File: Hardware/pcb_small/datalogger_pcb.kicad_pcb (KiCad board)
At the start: 2 copper layers, 127.5 x 123.3 mm, 45 parts, among them J1 Micro_SD_Card_Det2, J2 Switch OUT, SW1 SW_Wuerth_450301014042, U1 DS3231MZ

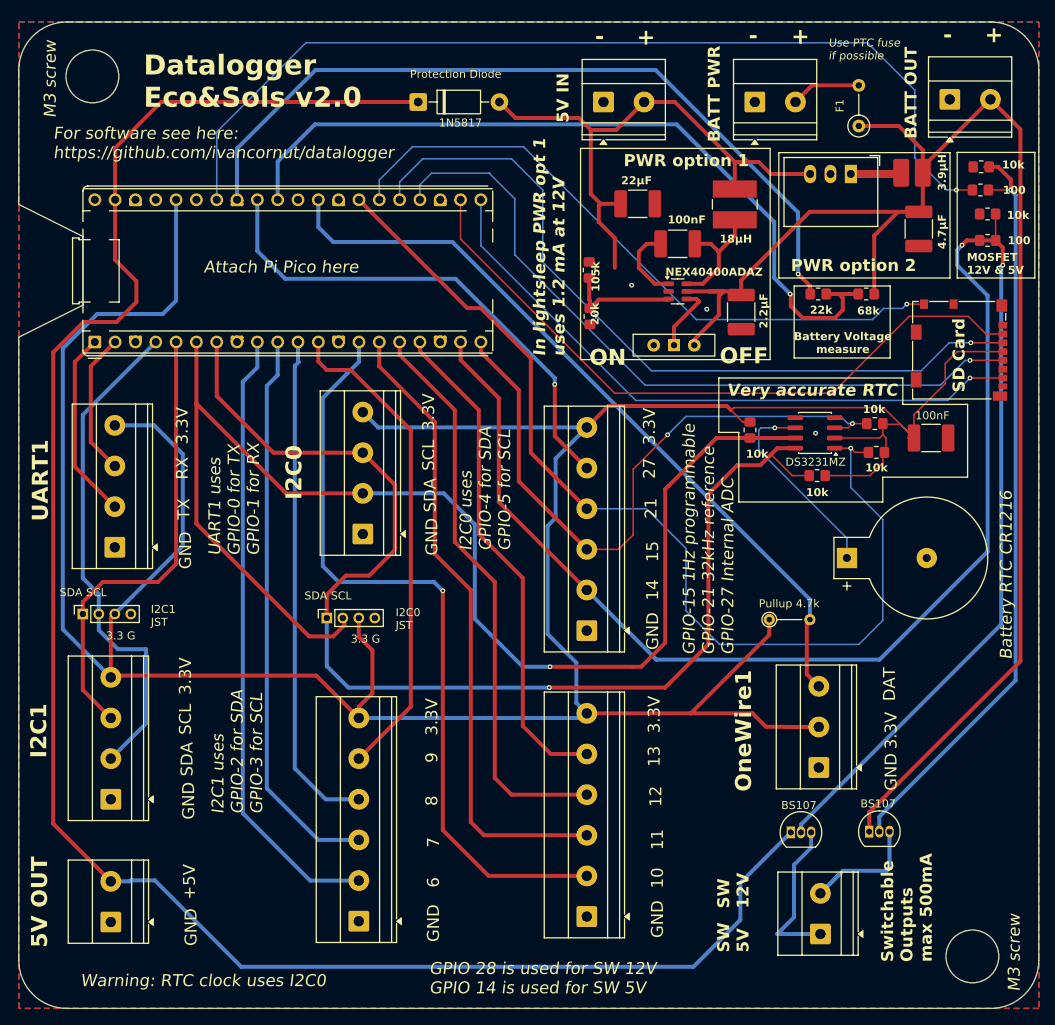
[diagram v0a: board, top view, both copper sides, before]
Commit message: Finalised design for micrologger
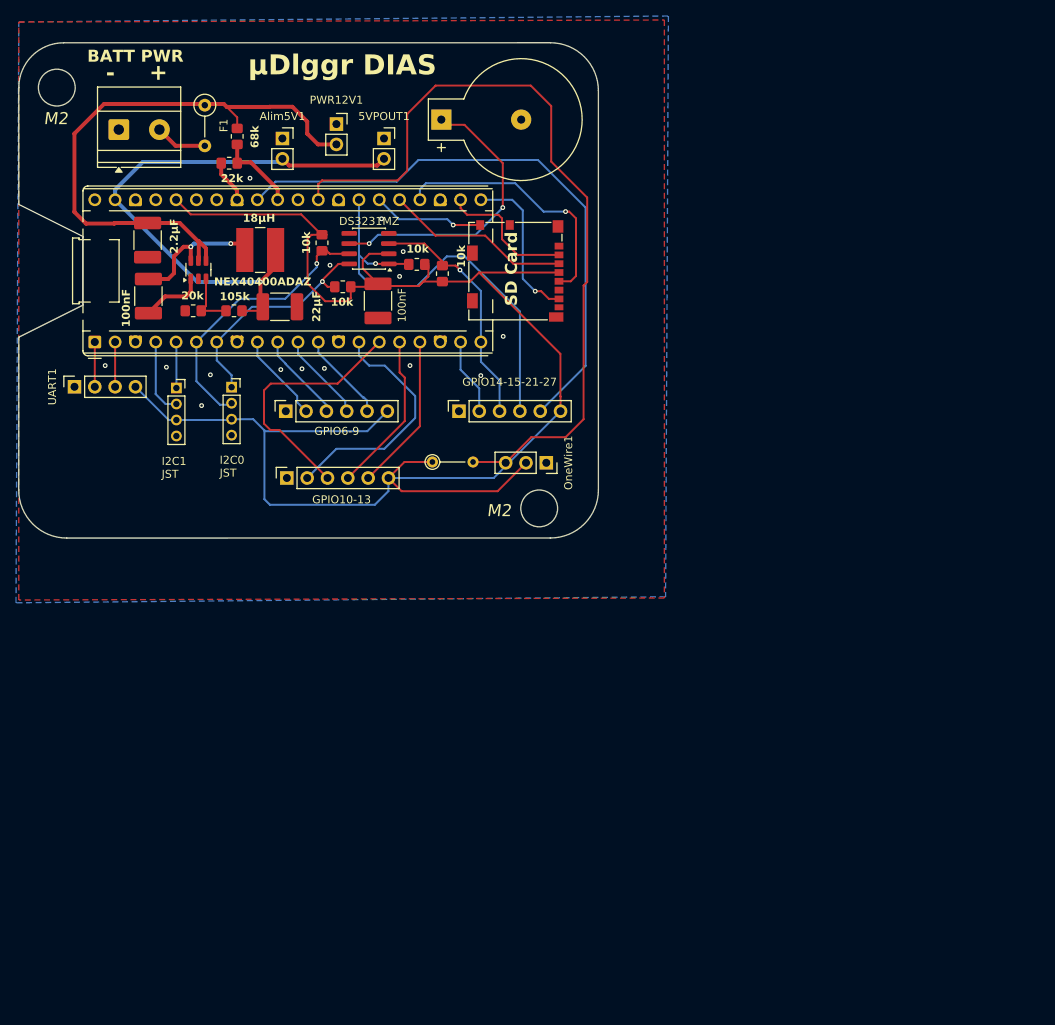
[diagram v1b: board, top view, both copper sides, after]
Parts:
- removed AlimOption2: R-78E5.0-0.5, Converter_DCDC:Converter_DCDC_RECOM_R-78E-0.5_THT
- removed C_alim2: 4.7 µF, Capacitor_SMD:C_1812_4532Metric_Pad1.57x3.40mm_HandSolder
- removed Diodeprotectionalim1: 1N5817, Diode_THT:D_DO-41_SOD81_P10.16mm_Horizontal
- removed I2C1: I2C 1 Connector, TerminalBlock_Phoenix:TerminalBlock_Phoenix_MKDS-1,5-4-5.08_1x04_P5.08mm_Horizontal
- removed I2C2: I2C 0 Connector, TerminalBlock_Phoenix:TerminalBlock_Phoenix_MKDS-1,5-4-5.08_1x04_P5.08mm_Horizontal
- removed J2: Switch OUT, TerminalBlock_Phoenix:TerminalBlock_Phoenix_MKDS-1,5-2-5.08_1x02_P5.08mm_Horizontal
- removed L_alim2: 3.9 µH, useful:RLS-397
- removed MOSFET_12V1, MOSFET_5V1: BS170, Package_TO_SOT_THT:TO-92_Inline
- removed R7, R8: R, Resistor_SMD:R_0805_2012Metric_Pad1.20x1.40mm_HandSolder
- removed R_pdown_MFET_1, R_pdown_MFET_2: 10k, Resistor_SMD:R_0805_2012Metric_Pad1.20x1.40mm_HandSolder
- removed SW1: SW_Wuerth_450301014042, Button_Switch_THT:SW_Slide-03_Wuerth-WS-SLTV_10x2.5x6.4_P2.54mm
- 5VPOUT1, Alim5V1, PWR12V1: footprint TerminalBlock_Phoenix:TerminalBlock_Phoenix_MKDS-1,5-2-5.08_1x02_P5.08mm_Horizontal -> Connector_PinSocket_2.54mm:PinSocket_1x02_P2.54mm_Vertical
- GPIO10-13: renamed from GPIO10-1; footprint TerminalBlock_Phoenix:TerminalBlock_Phoenix_MKDS-1,5-6-5.08_1x06_P5.08mm_Horizontal -> Connector_PinSocket_2.54mm:PinSocket_1x06_P2.54mm_Vertical
- GPIO14-15-21-27: renamed from GPIO14-1; footprint TerminalBlock_Phoenix:TerminalBlock_Phoenix_MKDS-1,5-6-5.08_1x06_P5.08mm_Horizontal -> Connector_PinSocket_2.54mm:PinSocket_1x06_P2.54mm_Vertical
- GPIO6-9: renamed from GPIO6-1; footprint TerminalBlock_Phoenix:TerminalBlock_Phoenix_MKDS-1,5-6-5.08_1x06_P5.08mm_Horizontal -> Connector_PinSocket_2.54mm:PinSocket_1x06_P2.54mm_Vertical
- OneWire1: footprint TerminalBlock_Phoenix:TerminalBlock_Phoenix_MKDS-1,5-3-5.08_1x03_P5.08mm_Horizontal -> Connector_PinSocket_2.54mm:PinSocket_1x03_P2.54mm_Vertical
- UART1: footprint TerminalBlock_Phoenix:TerminalBlock_Phoenix_MKDS-1,5-4-5.08_1x04_P5.08mm_Horizontal -> Connector_PinSocket_2.54mm:PinSocket_1x04_P2.54mm_Vertical
- moved 5VPOUT1 103.7 mm to (95.7, 42.6), turned to 0 degrees
- moved F1 81.8 mm to (73.2, 38.4), turned to -90 degrees
- moved R1 81.1 mm to (77.3, 42.3), turned to -90 degrees
- moved PWRIN1 79.6 mm to (62.5, 41.5)
- moved PWR12V1 76.7 mm to (89.7, 40.8)
- moved R2 75.4 mm to (76.3, 45.6)
- moved C2 74.7 mm to (66.1, 55.3)
- moved BT1 74.7 mm to (102.8, 40.2)
- moved C4 71.2 mm to (94.9, 62.9), turned to -90 degrees
- moved C1 66.5 mm to (66.2, 62.3), turned to 90 degrees
- moved GPIO10-13 66.4 mm to (83.5, 85.0)
- moved GPIO6-9 64.4 mm to (83.4, 76.7)
- moved Rpllup2 63.8 mm to (90.5, 61.1)
- moved R5 62.1 mm to (99.8, 58.3)
- moved U1 60.3 mm to (93.8, 56.3)
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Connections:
- 5VPOUT1 pad 2: +5VP -> +5V
- A1 pad 34: Net-(A1-GPIO28_ADC2) -> unconnected-(A1-GPIO28_ADC2-Pad34)
- A1 pad 39: +5VP -> +5V
- Alimoption1 pad 4: Net-(Alimoption1-EN) -> +12V
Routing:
- net +5VP: track 241.9 -> 0.00 mm
- net +3.3V: track 394.8 -> 208.1 mm
- net /I2C0_SDA: track 167.1 -> 35.3 mm
- net Net-(A1-GPIO14): track 139.1 -> 9.62 mm, vias 1 -> 0
- net /I2C0_SCL: track 150.4 -> 29.6 mm
- net Net-(A1-GPIO28_ADC2): track 120.1 -> 0.00 mm, vias 1 -> 0
- net +12V: track 184.8 -> 72.7 mm
- net Net-(MOSFET_12V1-G): track 95.5 -> 0.00 mm, vias 1 -> 0
- net /AGND: track 98.8 -> 5.39 mm, vias 1 -> 0
- net Net-(MOSFET_5V1-G): track 90.1 -> 0.00 mm, vias 1 -> 0
- net /READ12V: track 98.9 -> 10.2 mm, vias 1 -> 0
- net Net-(A1-GPIO21): track 128.9 -> 53.7 mm
- net /MOSI: track 96.5 -> 23.2 mm, vias 1 -> 0
- net /CS: track 85.6 -> 17.3 mm
- net /CD: track 82.0 -> 13.9 mm
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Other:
- board size 127.5 x 123.3 mm -> 72.5 x 61.9 mm
- board text added: "M2"
- board text added: "µDlggr DIAS"
- board text removed: "+5V"
- board text removed: "10"
- board text removed: "100"
- board text removed: "11"
- board text removed: "12"
- board text removed: "13"
- board text removed: "14"
- board text removed: "15"
- board text removed: "1N5817"
- board text removed: "21"
- board text removed: "27"
- board text removed: "3.3 G"
- board text removed: "3.3V"
- board text removed: "3.9µH"
- board text removed: "4.7µF"
- board text removed: "5V IN"
- board text removed: "5V OUT"
- board text removed: "6"
- board text removed: "7"
- board text removed: "8"
- board text removed: "9"
- board text removed: "Attach Pi Pico here"
- board text removed: "BATT OUT"
- board text removed: "BS107"
- board text removed: "Battery RTC CR1216"
- board text removed: "Battery Voltage measure"
- board text removed: "DAT"
- board text removed: "Datalogger Eco&Sols v2.0"
- board text removed: "For software see here: https://github.com/ivancornut/datalogger"
- board text removed: "GND"
- board text removed: "GPIO 28 is used for SW 12V GPIO 14 is used for SW 5V"
- board text removed: "GPIO-15 1Hz programmable GPIO-21 32kHz reference GPIO-27 Internal ADC"
- board text removed: "I2C0"
- board text removed: "I2C0 uses GPIO-4 for SDA GPIO-5 for SCL"
- board text removed: "I2C1 uses GPIO-2 for SDA GPIO-3 for SCL"
- board text removed: "In lightsleep PWR opt 1 uses 1.2 mA at 12V"
- board text removed: "M3 screw"
- board text removed: "MOSFET 12V & 5V"
- board text removed: "OFF"
- board text removed: "ON"
- board text removed: "PWR option 1"
- board text removed: "PWR option 2"
- board text removed: "Protection Diode"
- board text removed: "Pullup 4.7k"
- board text removed: "RX"
- board text removed: "SCL"
- board text removed: "SDA"
- board text removed: "SDA SCL"
- board text removed: "SW 12V"
- board text removed: "SW 5V"
- board text removed: "Switchable Outputs max 500mA"
- board text removed: "TX"
- board text removed: "UART1 uses GPIO-0 for TX GPIO-1 for RX"
- board text removed: "Use PTC fuse if possible"
- board text removed: "Very accurate RTC"
- board text removed: "Warning: RTC clock uses I2C0"
